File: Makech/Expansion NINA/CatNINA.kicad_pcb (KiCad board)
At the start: 2 copper layers, 62.9 x 33.4 mm, 25 parts, among them J1 Conn_02x03_Odd_Even, J2 Conn_02x03_Odd_Even, P3 PROGRAMMER SERIAL, P4 Battery, U1 ESP32-WROOM, U2 AP2112K-3.3TRG1, U3 MCP73831T-2ACI/OT

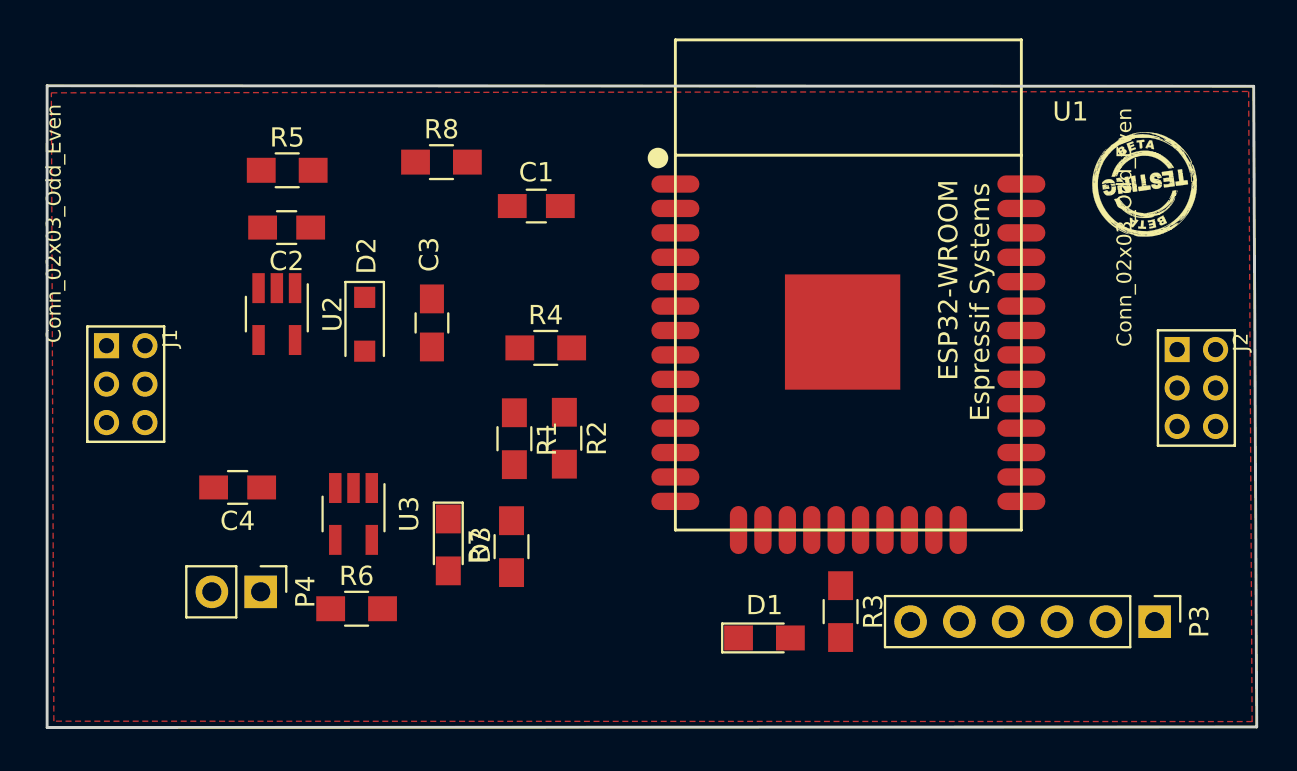
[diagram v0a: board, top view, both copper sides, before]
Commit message: Init PCB and netlist
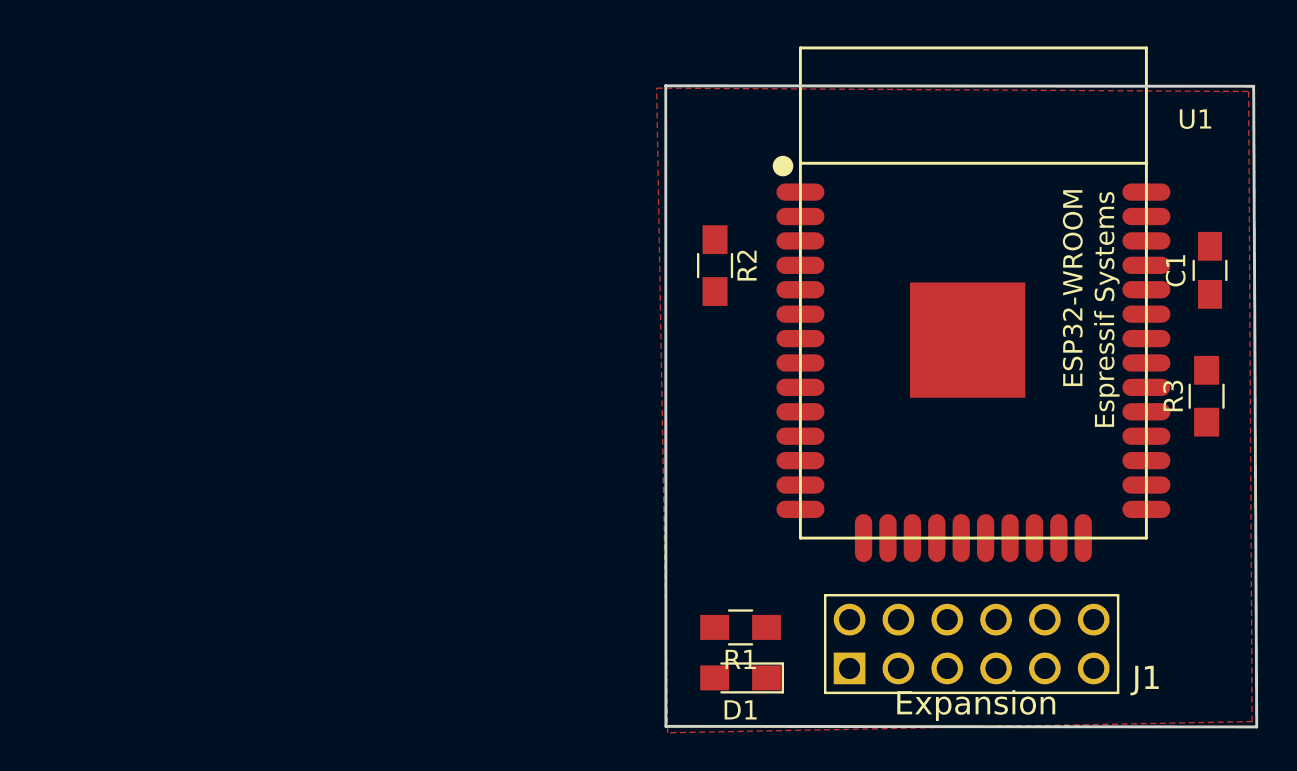
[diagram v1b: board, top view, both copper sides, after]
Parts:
- removed C2, C3, C4: 10uF, Capacitors_SMD:C_0805_HandSoldering
- removed D2: D_Schottky, Diodes_SMD:D_SOD-123F
- removed D3: LED, LEDs:LED_0805_HandSoldering
- removed J2: Conn_02x03_Odd_Even, Pines:62000621121
- removed P3: PROGRAMMER SERIAL, Pin_Headers:Pin_Header_Straight_1x06_Pitch2.54mm
- removed P4: Battery, Pin_Headers:Pin_Header_Straight_1x02_Pitch2.54mm
- removed R4, R5: 10k, Resistors_SMD:R_0805_HandSoldering
- removed R6: 1K, Resistors_SMD:R_0805_HandSoldering
- removed R7: 4.7K, Resistors_SMD:R_0805_HandSoldering
- removed R8: 10K, Resistors_SMD:R_0805_HandSoldering
- removed U2: AP2112K-3.3TRG1, TO_SOT_Packages_SMD:SOT-23-5_HandSoldering
- removed U3: MCP73831T-2ACI/OT, TO_SOT_Packages_SMD:SOT-23-5_HandSoldering
- G***: moved to B.Cu
- J1: value Conn_02x03_Odd_Even -> Expansion; footprint Pines:62000621121 -> Pines:61301221121
- R1: value 100k -> 330
- R2: value 100k -> 10k
- R3: value 330 -> 10K
- moved J1 46.0 mm to (193.8, 106.4), turned to 0 degrees
- moved C1 35.2 mm to (206.2, 86.9), turned to 90 degrees
- moved R3 22.1 mm to (206.0, 93.5), turned to 90 degrees
- moved G*** 15.8 mm to (190.4, 92.2), turned to 0 degrees
- moved R1 15.3 mm to (181.8, 105.5), turned to 180 degrees
- moved R2 11.9 mm to (180.5, 86.7)
- moved U1 6.52 mm to (193.9, 88.1)
- moved G*** 6.16 mm to (201.6, 87.3)
- moved D1 2.42 mm to (181.8, 108.1), turned to 180 degrees
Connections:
- J1 pad 1: /MOSI -> /ESP_TX
- J1 pad 2: /MISO -> +3V3
- J1 pad 3: /SCK -> /ESP_RX
- J1 pad 4: /ESP_GPIO0 -> /ESP_BUSY
- J1 pad 5: /ESP_RESET -> /ESP_CS
- J1 pad 6: VCC -> /ESP_RTS
- R1 pad 1: +BATT -> /IO25
- R1 pad 2: /AN35_BAT -> Net-(D1-Pad2)
- R2 pad 1: /AN35_BAT -> /ESP_RESET
- R3 pad 1: /IO25 -> +3V3
- R3 pad 2: Net-(D1-Pad2) -> /ESP_CS
- U1 pad 13: /MOSI -> /ESP_MOSI
- U1 pad 30: /SCK -> /ESP_SCK
- U1 pad 37: /MISO -> /ESP_MISO
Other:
- board size 62.9 x 33.4 mm -> 30.7 x 33.4 mm
- board text added: "CatNINA"
- board text removed: "Backpack BLE"

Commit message: size in margin
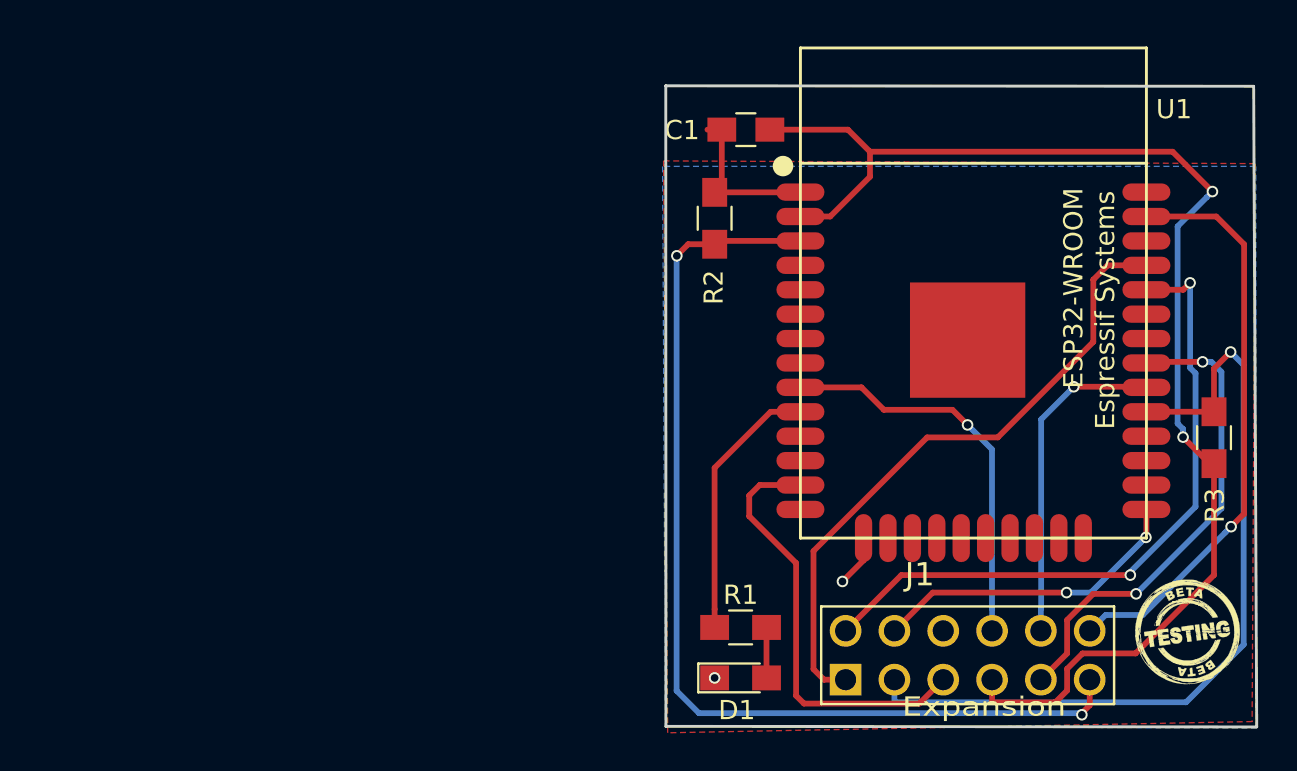
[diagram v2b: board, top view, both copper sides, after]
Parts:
- removed the G*** at (195.7, 80.4)
- added G***: LOGO, Aesthetics:escornabot_8x8, B.Cu at (184.5, 94.9)
- G***: moved to F.Cu
- moved C1 25.2 mm to (182.1, 79.6), turned to 180 degrees
- moved G*** 20.0 mm to (205.0, 105.8)
- moved G*** 9.24 mm to (200.7, 96.5)
- moved R2 2.46 mm to (180.4, 84.2), turned to 90 degrees
- moved R3 2.19 mm to (206.4, 95.6)
- moved J1 0.62 mm to (193.6, 106.9)
- turned D1 to 0 degrees
- turned R1 to 0 degrees
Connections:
- J1 pad 10: /ESP_RESET -> /ESP_SCK
- J1 pad 11: GND -> /ESP_RESET
- J1 pad 2: +3V3 -> /ESP_RX
- J1 pad 3: /ESP_RX -> /ESP_CS
- J1 pad 4: /ESP_BUSY -> /ESP_GPIO0
- J1 pad 5: /ESP_CS -> /ESP_MOSI
- J1 pad 6: /ESP_RTS -> GND
- J1 pad 7: /ESP_GPIO0 -> +3V3
- J1 pad 8: /ESP_SCK -> /ESP_BUSY
- J1 pad 9: /ESP_MOSI -> /ESP_RTS
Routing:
- net +3V3: track 0.00 -> 67.9 mm, vias 0 -> 2
- net /ESP_RESET: track 0.00 -> 53.0 mm, vias 0 -> 2
- net /ESP_CS: track 0.00 -> 43.1 mm, vias 0 -> 1
- net /ESP_RX: track 0.00 -> 35.2 mm, vias 0 -> 2
- net /ESP_TX: track 0.00 -> 33.4 mm
- net /ESP_MISO: track 0.00 -> 30.3 mm, vias 0 -> 1
- net /ESP_RTS: track 0.00 -> 25.4 mm, vias 0 -> 2
- net /ESP_MOSI: track 0.00 -> 22.7 mm
- net /ESP_BUSY: track 0.00 -> 20.7 mm, vias 0 -> 1
- net /ESP_SCK: track 0.00 -> 17.2 mm, vias 0 -> 1
- net /ESP_GPIO0: track 0.00 -> 16.6 mm, vias 0 -> 2
- net /IO25: track 0.00 -> 14.0 mm
- net GND: track 0.00 -> 11.3 mm, vias 0 -> 2
- net Net-(D1-Pad2): track 0.00 -> 2.63 mm
- added copper zone on B.Cu, net GND
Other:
- board text added: "Co-Processor"
- board text added: "ESP32 WIFI & BLE"
- board text added: "Escornabot Makech"
- board text added: "SPI Interface"
- board text added: "v0.1"
